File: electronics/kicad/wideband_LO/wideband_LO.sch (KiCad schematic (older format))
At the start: 49 parts, among them J1 CONN_06SMD, Q1 2N7002, Q2 BSS84, Q3 BSS84, U1 BFP620

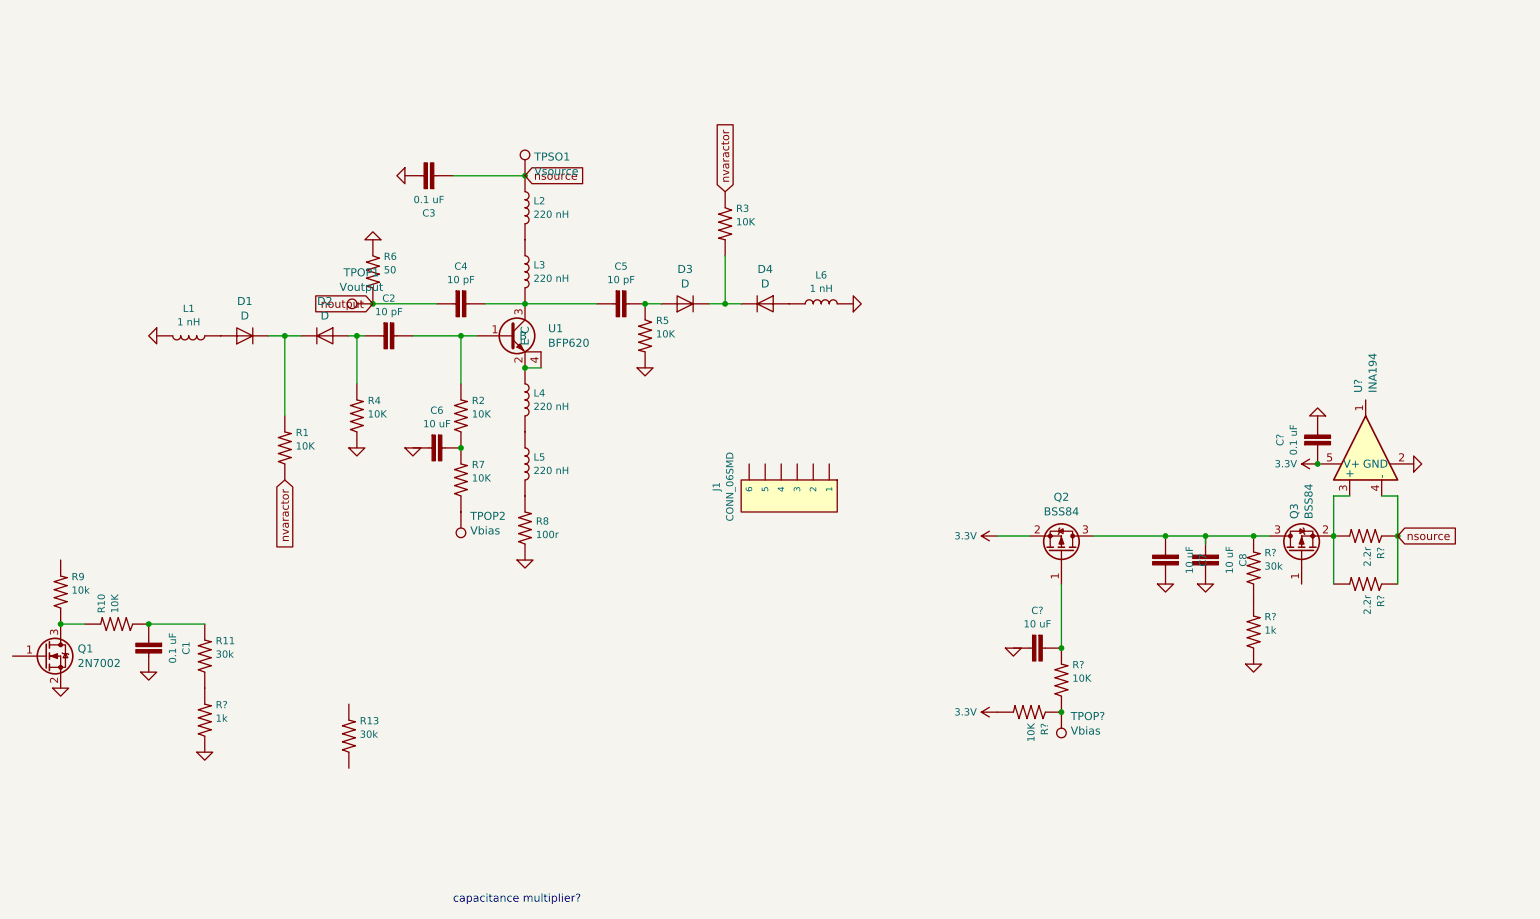
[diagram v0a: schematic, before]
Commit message: Backup
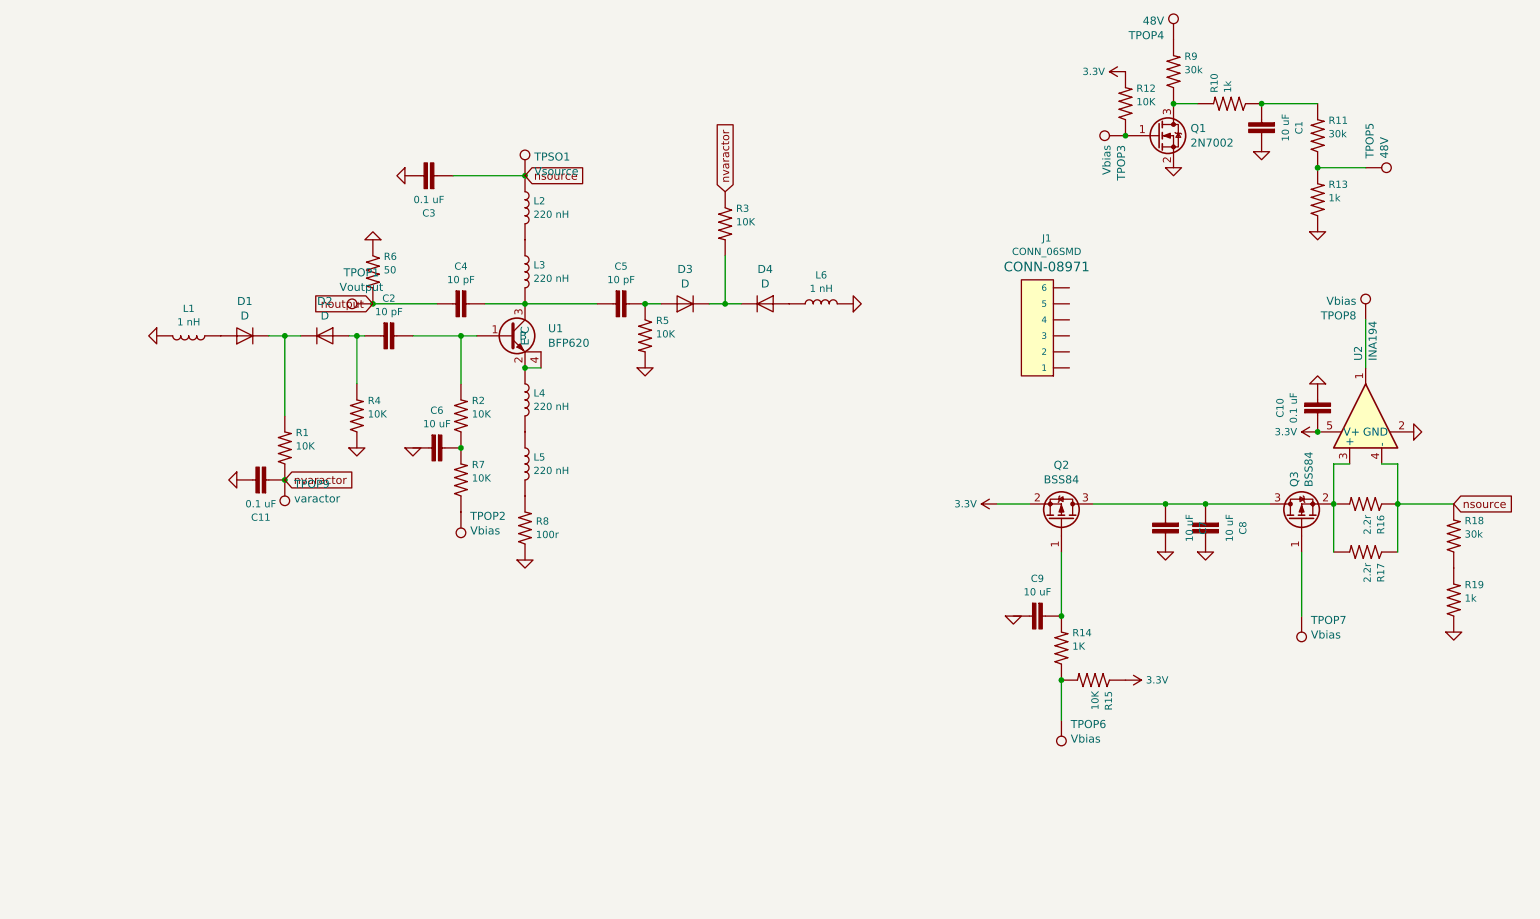
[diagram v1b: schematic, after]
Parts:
- removed R13: 30k, Resistor_SMD:R_0402_1005Metric, symbol SparkFun-Resistors:RESISTOR0402
- added C11: 0.1 uF, 0603, symbol SparkFun-Capacitors:4.7UF0603
- added R12: 10K, Resistor_SMD:R_0402_1005Metric, symbol SparkFun-Resistors:RESISTOR0402
- added TPOP3, TPOP7, TPOP8: Vbias, TestPoint:TestPoint_Pad_1.5x1.5mm, symbol Connector:Test_Point
- added TPOP4, TPOP5: 48V, TestPoint:TestPoint_Pad_1.5x1.5mm, symbol Connector:Test_Point
- added TPOP9: varactor, TestPoint:TestPoint_Pad_1.5x1.5mm, symbol Connector:Test_Point
- C1: value 0.1 uF -> 10 uF
- J1: Field4 (none) -> CONN-08971
- R10: value 10K -> 1k
- R14: renamed from R?; value 10K -> 1K
- R9: value 10k -> 30k
- gave numbers to parts that had none: 10
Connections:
- wire segments 33 -> 36
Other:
- note removed: "capacitance multiplier?\n"
- moved on the sheet: C10, C7, C8, C9, Q1, Q2, Q3, R10, R11, R13, R14, R15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
